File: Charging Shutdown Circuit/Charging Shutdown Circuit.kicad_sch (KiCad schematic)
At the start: 38 parts, among them J1 IMD, J2 Shutdown IL, J3 776087-1, J4 776087-1, K1 Latching Relay, K4 GIGAVAC GX14BAB, K5 GIGAVAC GX14BB, Q1 STS6NF20V, SW1 SW-STOP, SW2 SH_RESET, U1 DK1A1B-12V, U10 NAND, U11 LM555N, U3 NSL-32, U4 NSL-32, U5 DK1A1B-12V, U6 NSL-32, U7 NSL-32, U8 DK1A1B-12V, U9 NSL-32

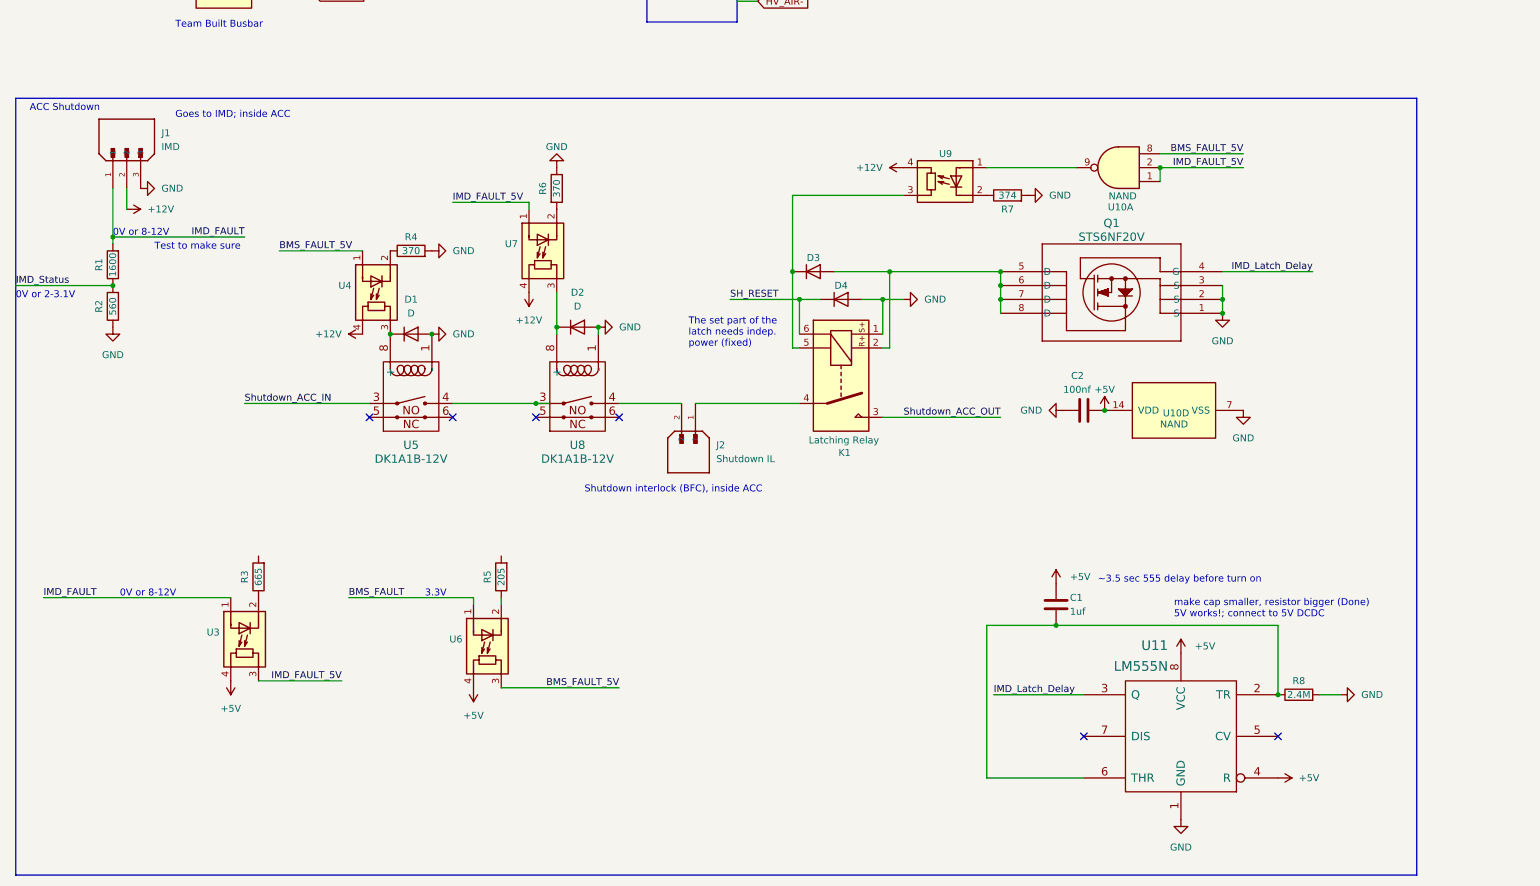
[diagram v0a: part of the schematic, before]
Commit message: charger stuff (don't break plz)
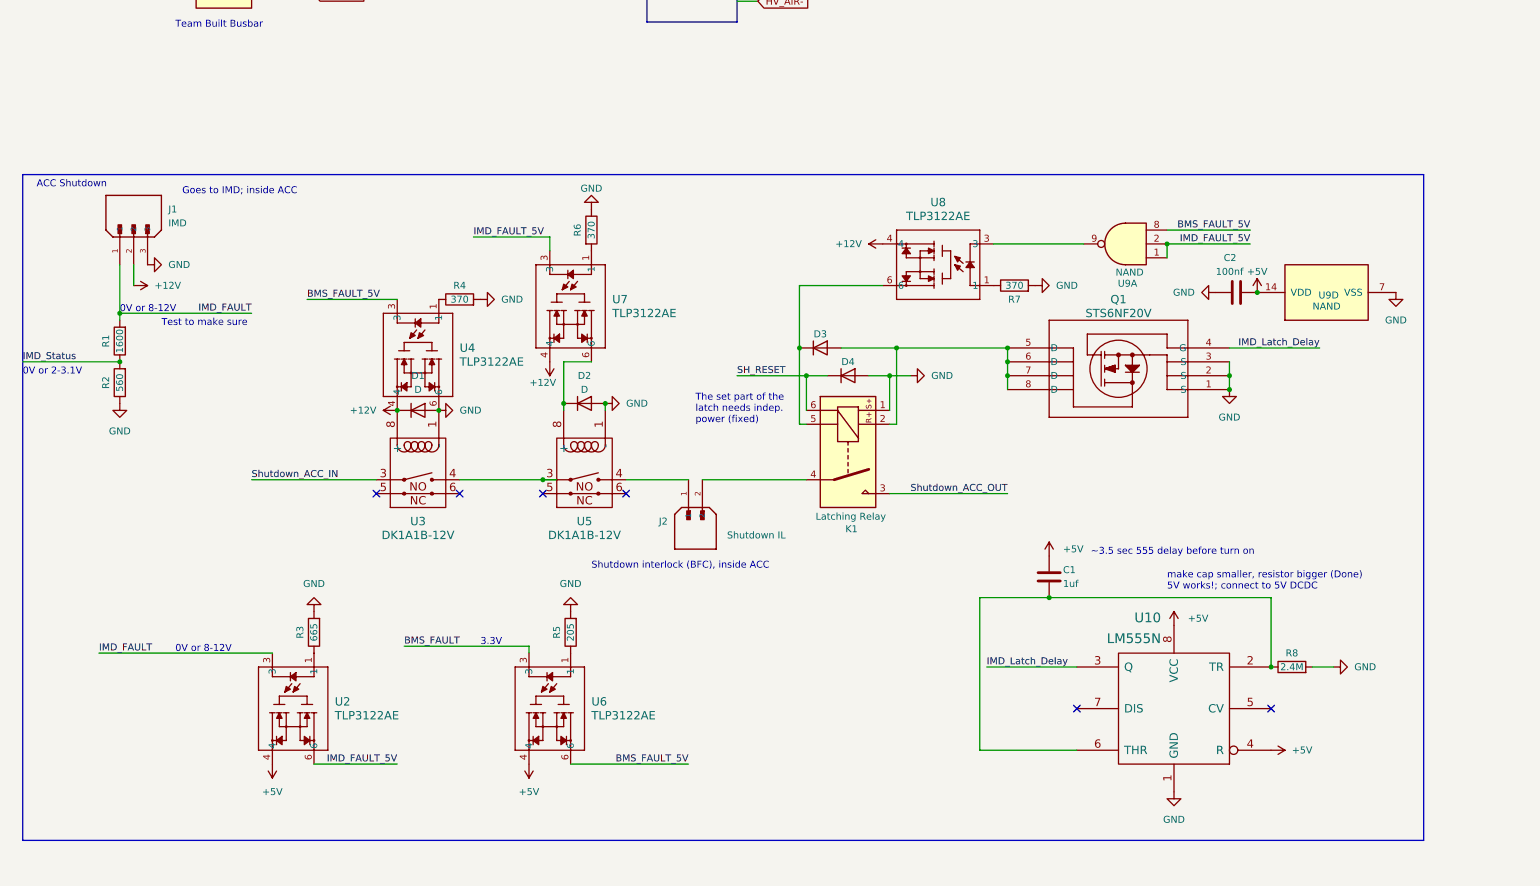
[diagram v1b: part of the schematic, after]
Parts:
- removed U10: NAND, Package_DIP:DIP-14_W7.62mm, symbol 4xxx:4023
- removed U11: LM555N, Package_DIP:DIP-8_W7.62mm, symbol 2FS-1_Symbol Library:LM555N
- removed U3, U4, U6, U7, U9: NSL-32, 1FS_2_Global_Footprint_Library:OptoCoupler 6-SOP, symbol Isolator:NSL-32
- removed U8: DK1A1B-12V, 1FS_2_Global_Footprint_Library:RELAY_DK2A_PAN, symbol 2FS-1_Symbol Library:DK1A1B-12V
- added U10: LM555N, Package_DIP:DIP-8_W7.62mm, symbol 2FS-1_Symbol Library:LM555N
- added U2, U4, U6, U7, U8: TLP3122AE, 1FS_2_Global_Footprint_Library:OptoCoupler 6-SOP, symbol 1FS_2_Global_Symbol_Library:TLP3122AE
- added U3: DK1A1B-12V, 1FS_2_Global_Footprint_Library:RELAY_DK2A_PAN, symbol 2FS-1_Symbol Library:DK1A1B-12V
- added U9: NAND, Package_DIP:DIP-14_W7.62mm, symbol 4xxx:4023
- R7: value 374 -> 370
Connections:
- net +12V: now also D1.1 (K), U3.8 (+), U4.4, U7.4, U8.4
- net +5V: now also U10.4 (R), U10.8 (VCC), U2.4, U6.4, U9.14 (VDD)
- net BMS_FAULT: now also U6.3
- net BMS_FAULT_5V: now also U4.3, U6.6, U9.8
- net GND: now also R3.2, R5.2, U10.1 (GND), U3.1 (-), U4.6, U9.7 (VSS)
- net IMD_FAULT: now also U2.3
- net IMD_FAULT_5V: now also U2.6, U7.3, U9.1, U9.2
- net IMD_Latch_Delay: now also U10.3 (Q)
- net Shutdown_ACC_IN: now also U3.3; no longer U5.3
- net at R6.2: now also U7.1
- net at D2.1 (K): now also U5.8 (+), U7.6
- net at U5.4: now also J2.1
- net at R3.1: now also U2.1
- net at R5.1: now also U6.1
- net at J2.2: now also K1.4
- net at C1.2, R8.1: now also U10.2 (TR), U10.6 (THR)
- net at R7.1: now also U8.1
- net at D3.1 (K), K1.5: now also U8.6
- net at R4.1: now also U4.1
- new net: U3.4, U5.3
- new net: U8.3, U9.9
